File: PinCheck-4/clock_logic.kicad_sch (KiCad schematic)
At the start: 14 parts, among them J1 BatteryHolder, Q1 PMOS, SW1 SW_SPST, U1 TPS61221DCK, U2 ICM7555xB

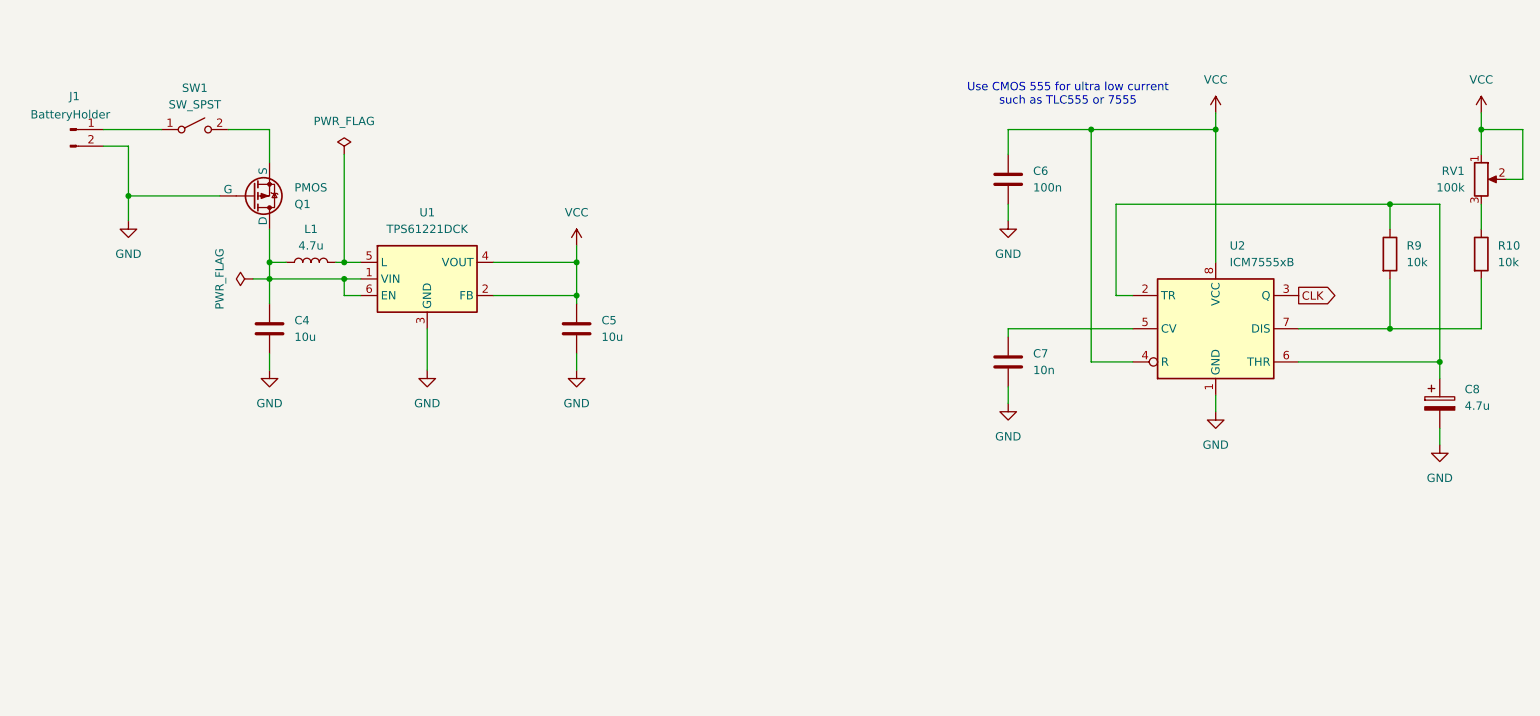
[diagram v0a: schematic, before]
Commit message: Daily sync 2025-08-30 13:49
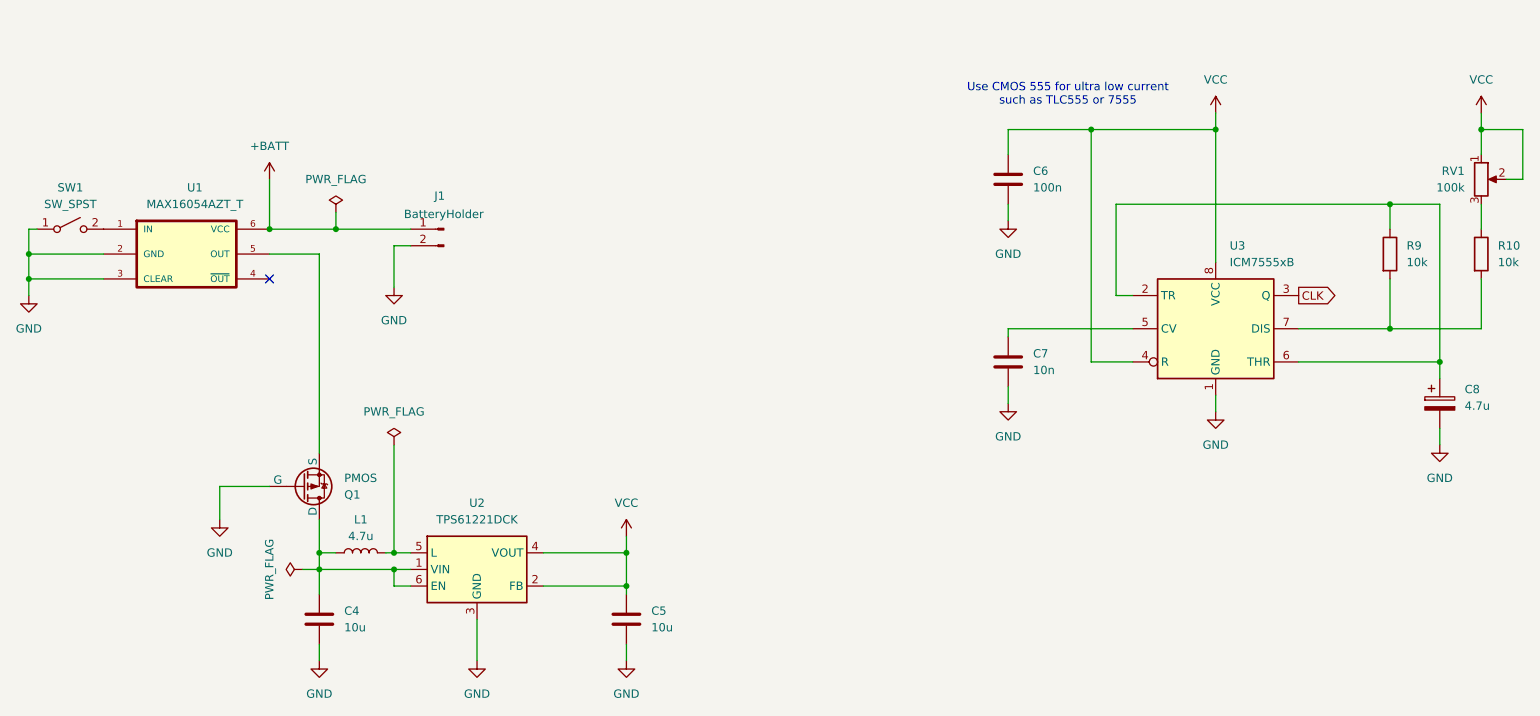
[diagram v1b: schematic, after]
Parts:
- added U1: MAX16054AZT_T, Package_TO_SOT_SMD:TSOT-23-6_HandSoldering, symbol Switch:MAX16054AZT_T
- SW1: footprint Button_Switch_THT:SW_DIP_SPSTx01_Slide_9.78x4.72mm_W7.62mm_P2.54mm -> Button_Switch_THT:SW_PUSH_6mm; Manufacturer Part No Dip Switch SPST 1 Position Through Hole Slide (Standard) Ac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 -> TS02-66-70-BK-260-LCR-D
- renumbered U1 to U2, U2 to U3
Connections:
- net GND: now also SW1.1 (A), U1.2 (GND), U1.3 (CLEAR)
- net at Q1.2 (S): now also U1.5 (OUT); no longer SW1.2 (B)
- net +BATT: now reaches J1.1 (Pin_1)
- net +BATT: now also U1.6 (VCC); no longer SW1.1 (A)
- new net: SW1.2 (B), U1.1 (IN)
- no-connect marks 0 -> 1
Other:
- moved on the sheet: C4, C5, J1, L1, Q1, SW1, U2

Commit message: Daily sync 2025-08-30 21:30
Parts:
- SW1: footprint Button_Switch_THT:SW_PUSH_6mm -> Button_Switch_SMD:SW_SPST_PTS645Sx43SMTR92; Manufacturer Part No TS02-66-70-BK-260-LCR-D -> TS04-66-70-BK-160-SMT
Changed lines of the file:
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@@
 			)
 		)
-		(property "Footprint" "Button_Switch_THT:SW_PUSH_6mm"
+		(property "Footprint" "Button_Switch_SMD:SW_SPST_PTS645Sx43SMTR92"
 			(at 36.83 93.98 0)
 			(effects
@@
 			)
 		)
-		(property "Description" "Tactile Switch SPST-NO Top Actuated Through Hole"
+		(property "Description" "TS04-66-70-BK-160-SMT"
 			(at 36.83 93.98 0)
 			(effects
@@
 			)
 		)
-		(property "Manufacturer Part No" "TS02-66-70-BK-260-LCR-D"
+		(property "Manufacturer Part No" "TS04-66-70-BK-160-SMT"
 			(at 36.83 93.98 0)
 			(effects

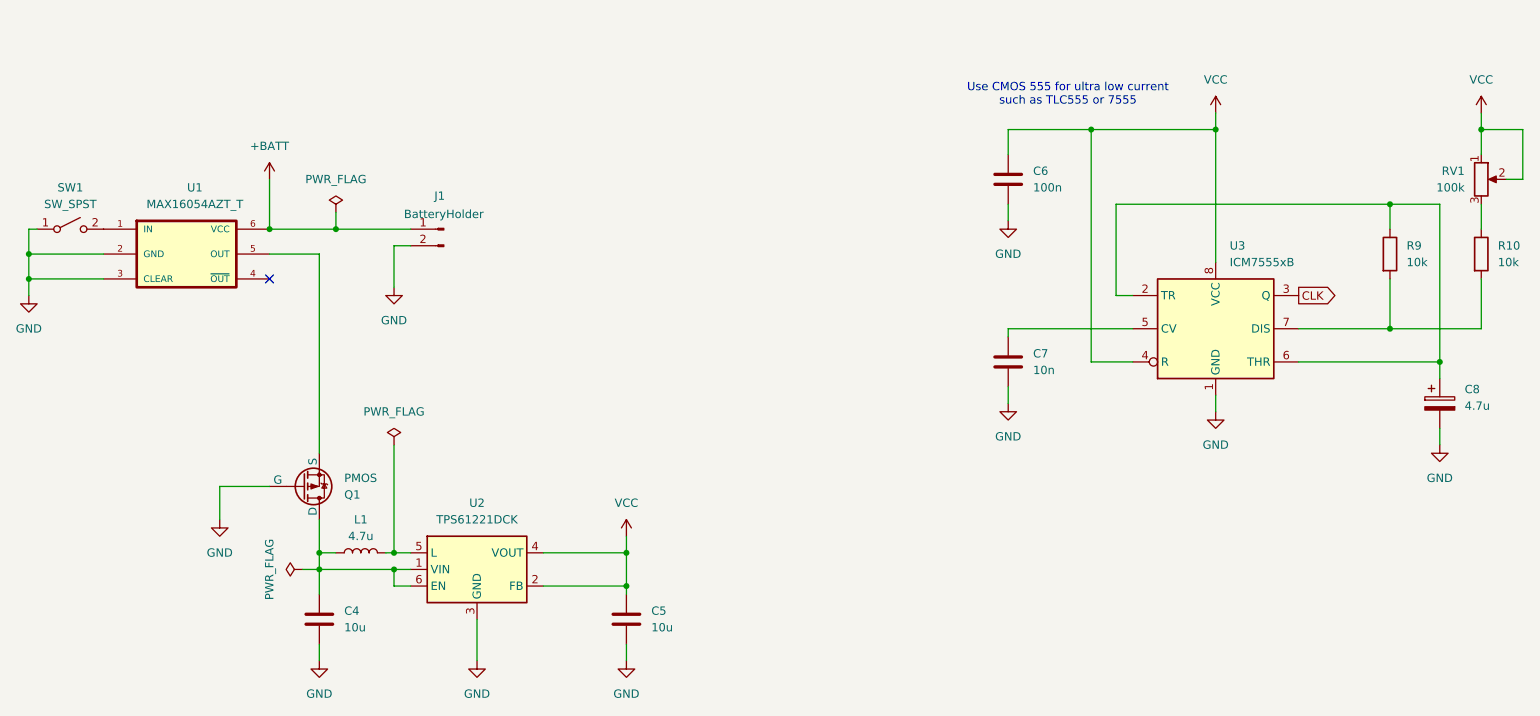
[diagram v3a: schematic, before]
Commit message: Daily sync 2025-09-01 09:07
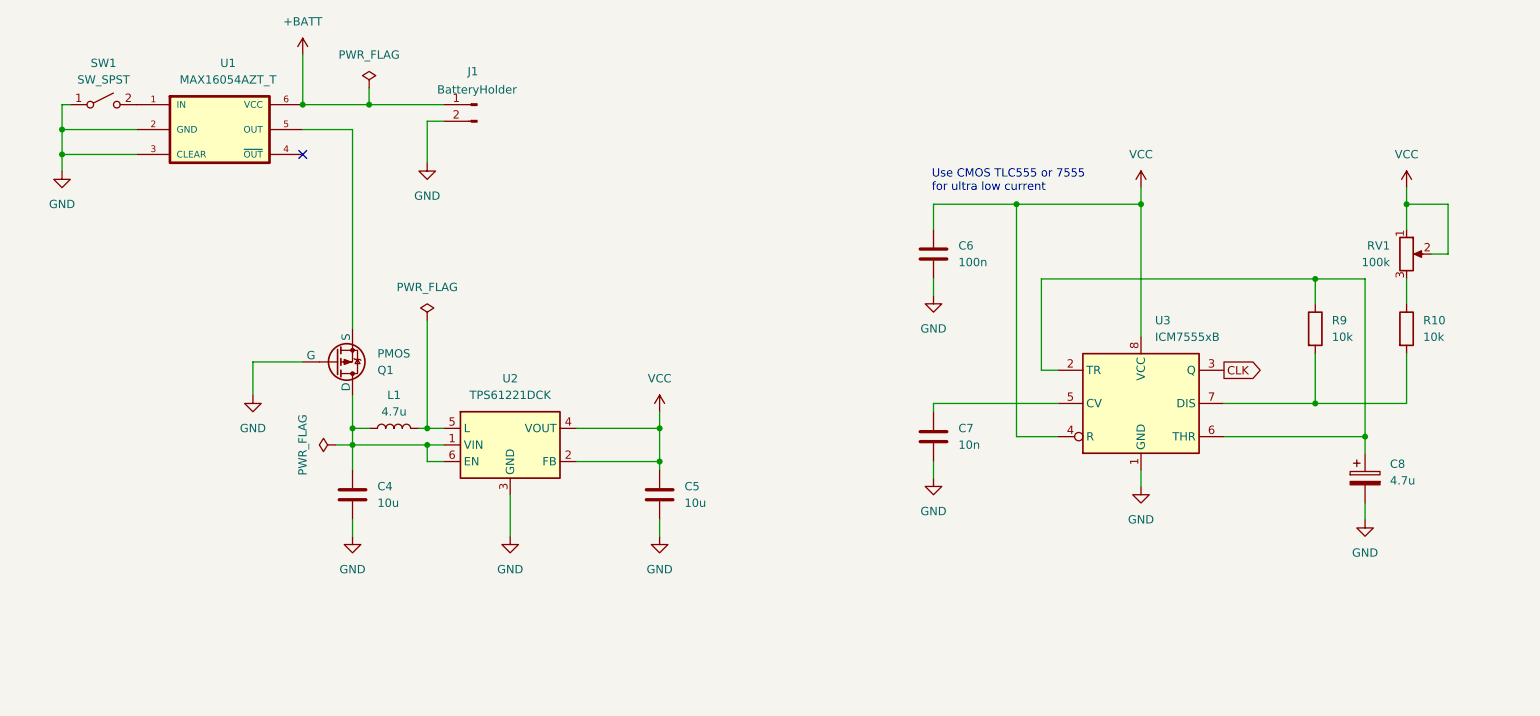
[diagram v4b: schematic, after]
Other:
- note added: "Use CMOS TLC555 or 7555 for ultra low current"
- note removed: "Use CMOS 555 for ultra low current such as TLC555 or 7555"
- moved on the sheet: C4, C5, C6, C7, C8, J1, L1, Q1, R10, R9, RV1, SW1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
